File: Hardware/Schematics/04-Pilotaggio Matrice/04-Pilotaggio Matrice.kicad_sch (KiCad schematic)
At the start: 10 parts, among them U1 CD74HC4067M, U2 CD74HC4067M, U3 CD74HC4067M, U69A AD8604ARUZ

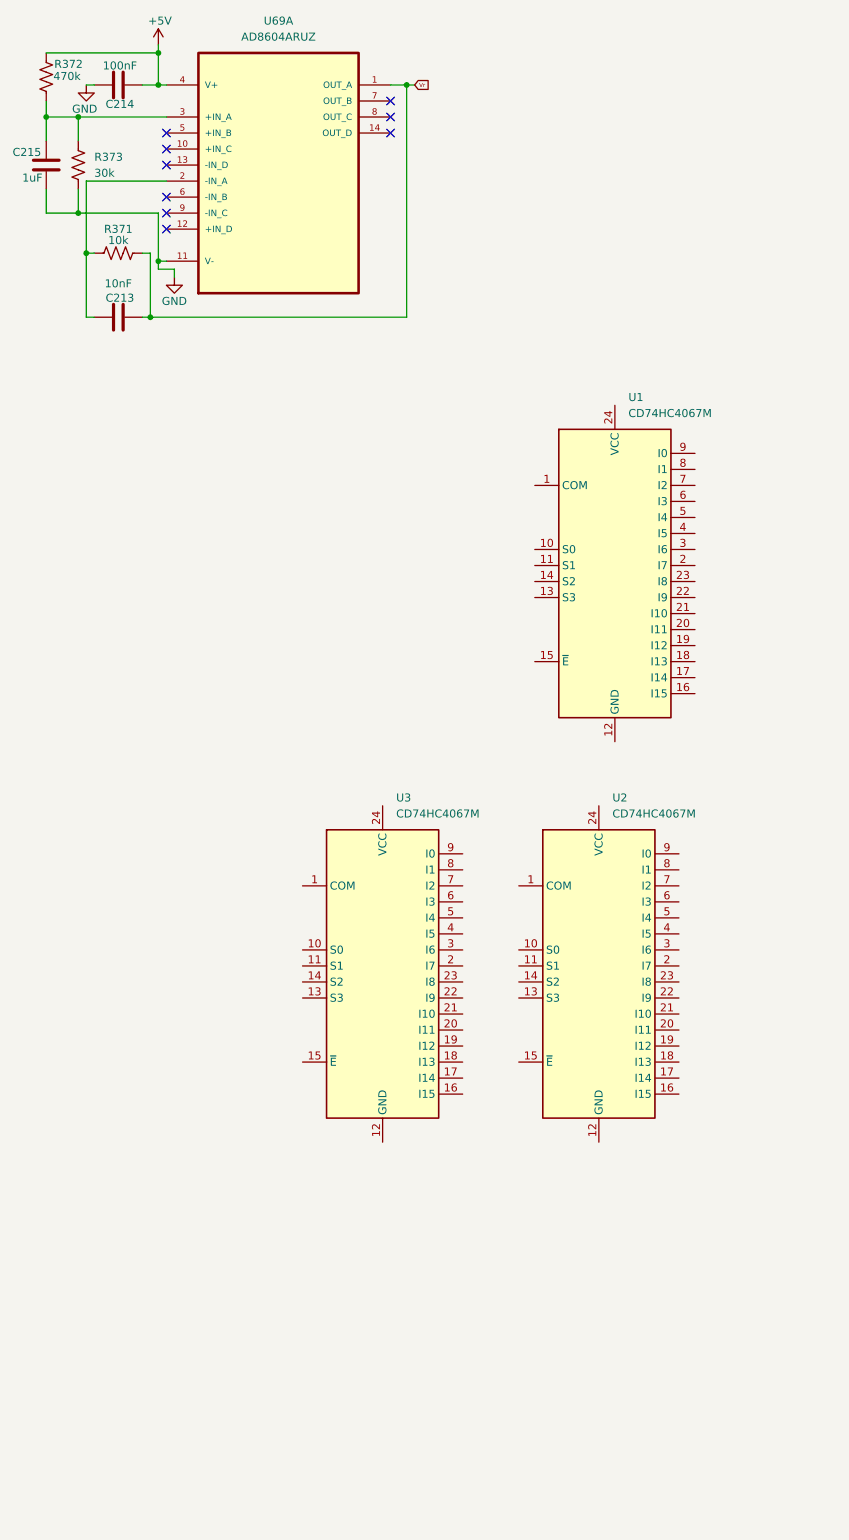
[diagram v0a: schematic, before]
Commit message: update
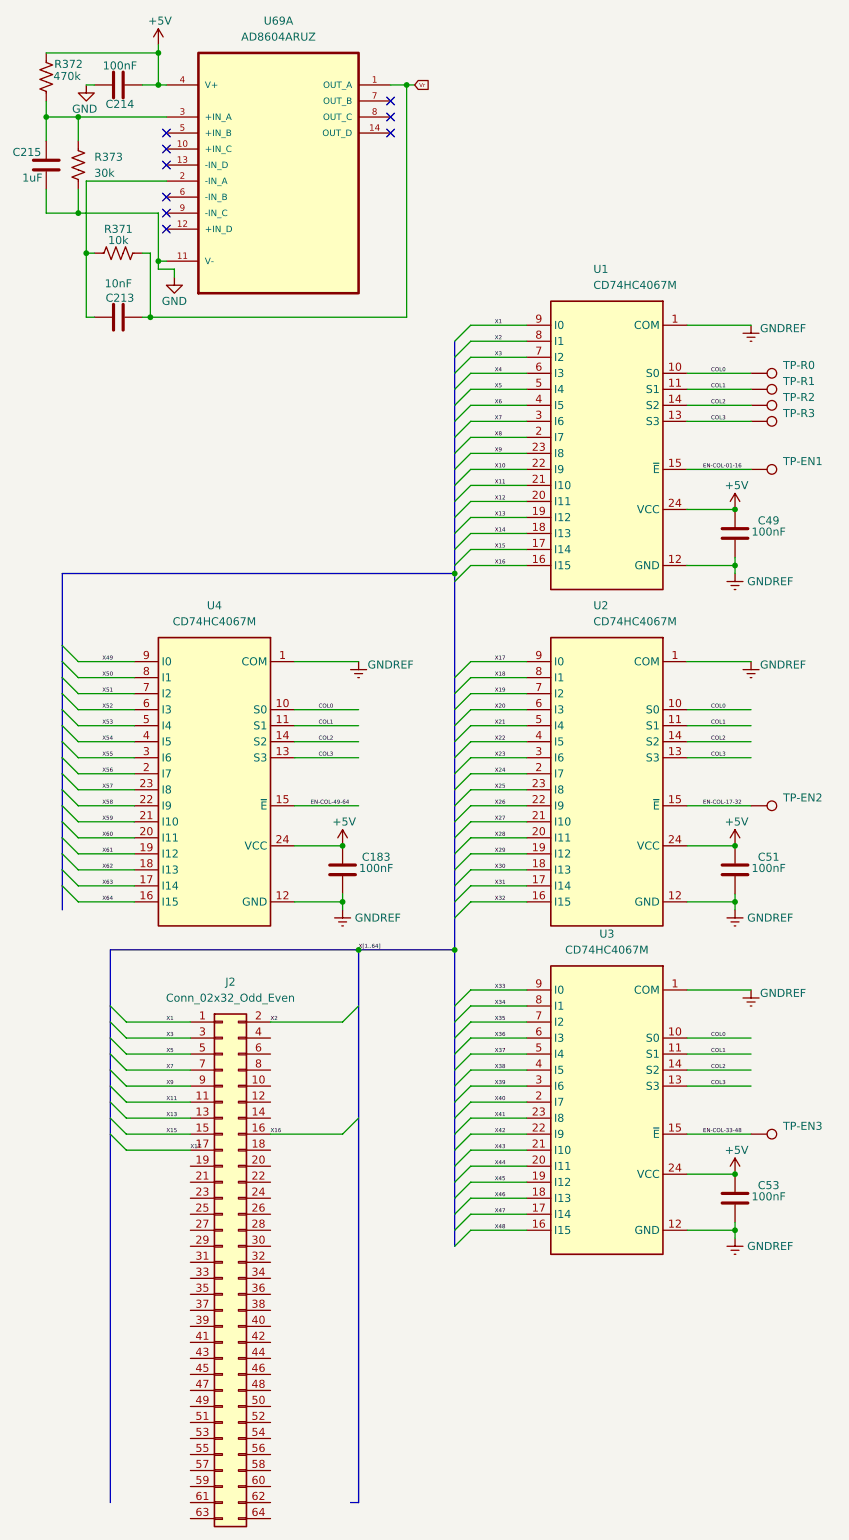
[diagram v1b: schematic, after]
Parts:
- added C183, C49, C51, C53: 100nF, symbol Device:C
- added J2: Conn_02x32_Odd_Even, Connector_PinHeader_1.00mm:PinHeader_2x32_P1.00mm_Vertical, symbol Connector_Generic:Conn_02x32_Odd_Even
- added TP-EN1, TP-EN2, TP-EN3, TP-R0, TP-R1, TP-R2, TP-R3: TestPoint, symbol Connector:TestPoint
- added U4: CD74HC4067M, Package_SO:SOIC-24W_7.5x15.4mm_P1.27mm, symbol 74xx:CD74HC4067M
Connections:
- net +5V: now also U1.24 (VCC), U2.24 (VCC), U3.24 (VCC), C183.2, C49.2, C51.2, C53.2, U4.24 (VCC)
- net GNDREF: now reaches U1.1 (COM)
- net GNDREF: now also U1.12 (GND), U2.1 (COM), U2.12 (GND), U3.1 (COM), U3.12 (GND), C183.1, C49.1, C51.1, C53.1, U4.1 (COM), U4.12 (GND)
- net COL0: now reaches U1.10 (S0)
- net COL0: now also U2.10 (S0), U3.10 (S0), TP-R0.1, U4.10 (S0)
- net COL1: now reaches U1.11 (S1)
- net COL1: now also U2.11 (S1), U3.11 (S1), TP-R1.1, U4.11 (S1)
- net COL3: now reaches U1.13 (S3)
- net COL3: now also U2.13 (S3), U3.13 (S3), TP-R3.1, U4.13 (S3)
- net COL2: now reaches U1.14 (S2)
- net COL2: now also U2.14 (S2), U3.14 (S2), TP-R2.1, U4.14 (S2)
- net EN-COL-01-16: now reaches U1.15 (~{E})
- net EN-COL-01-16: now also TP-EN1.1
- net X16: now reaches U1.16 (I15)
- net X16: now also J2.16 (Pin_16)
- net X15: now reaches U1.17 (I14)
- net X15: now also J2.15 (Pin_15)
- net X14: now reaches U1.18 (I13)
- net X13: now reaches U1.19 (I12)
- net X13: now also J2.13 (Pin_13)
- net X8: now reaches U1.2 (I7)
- net X12: now reaches U1.20 (I11)
- net X11: now reaches U1.21 (I10)
- net X11: now also J2.11 (Pin_11)
- net X10: now reaches U1.22 (I9)
- net X9: now reaches U1.23 (I8)
- net X9: now also J2.9 (Pin_9)
- net X7: now reaches U1.3 (I6)
- net X7: now also J2.7 (Pin_7)
- net X6: now reaches U1.4 (I5)
- net X5: now reaches U1.5 (I4)
- net X5: now also J2.5 (Pin_5)
- net X4: now reaches U1.6 (I3)
- net X3: now reaches U1.7 (I2)
- net X3: now also J2.3 (Pin_3)
- net X2: now reaches U1.8 (I1)
- net X2: now also J2.2 (Pin_2)
- net X1: now reaches U1.9 (I0)
- net X1: now also J2.1 (Pin_1)
- net EN-COL-17-32: now reaches U2.15 (~{E})
- net EN-COL-17-32: now also TP-EN2.1
- net X32: now reaches U2.16 (I15)
- net X31: now reaches U2.17 (I14)
- net X30: now reaches U2.18 (I13)
- net X29: now reaches U2.19 (I12)
- net X24: now reaches U2.2 (I7)
- net X28: now reaches U2.20 (I11)
- net X27: now reaches U2.21 (I10)
- net X26: now reaches U2.22 (I9)
- net X25: now reaches U2.23 (I8)
- net X23: now reaches U2.3 (I6)
- net X22: now reaches U2.4 (I5)
- net X21: now reaches U2.5 (I4)
- net X20: now reaches U2.6 (I3)
- net X19: now reaches U2.7 (I2)
- net X18: now reaches U2.8 (I1)
- net X17: now reaches U2.9 (I0)
- net X17: now also J2.17 (Pin_17)
- net EN-COL-33-48: now reaches U3.15 (~{E})
- net EN-COL-33-48: now also TP-EN3.1
- net X48: now reaches U3.16 (I15)
- net X47: now reaches U3.17 (I14)
- net X46: now reaches U3.18 (I13)
- net X45: now reaches U3.19 (I12)
- net X40: now reaches U3.2 (I7)
- net X44: now reaches U3.20 (I11)
- net X43: now reaches U3.21 (I10)
- net X42: now reaches U3.22 (I9)
- net X41: now reaches U3.23 (I8)
- net X39: now reaches U3.3 (I6)
- net X38: now reaches U3.4 (I5)
- net X37: now reaches U3.5 (I4)
- net X36: now reaches U3.6 (I3)
- net X35: now reaches U3.7 (I2)
- net X34: now reaches U3.8 (I1)
- net X33: now reaches U3.9 (I0)
- new net EN-COL-49-64: U4.15 (~{E})
- new net X49: U4.9 (I0)
- new net X50: U4.8 (I1)
- new net X51: U4.7 (I2)
- new net X52: U4.6 (I3)
- new net X53: U4.5 (I4)
- new net X54: U4.4 (I5)
- new net X55: U4.3 (I6)
- new net X56: U4.2 (I7)
- new net X57: U4.23 (I8)
- new net X58: U4.22 (I9)
- new net X59: U4.21 (I10)
- new net X60: U4.20 (I11)
- new net X61: U4.19 (I12)
- new net X62: U4.18 (I13)
- new net X63: U4.17 (I14)
- new net X64: U4.16 (I15)
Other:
- moved on the sheet: U1
